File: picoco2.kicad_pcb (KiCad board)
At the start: 2 copper layers, 53.3 x 93.2 mm, 19 parts, among them J1 Conn_01x03_Female, Q1 Q_NMOS_GDS, SW1 SW_Push, SW2 SW_Push, U1 PicoW, U2 scd30, U3 ssd1306

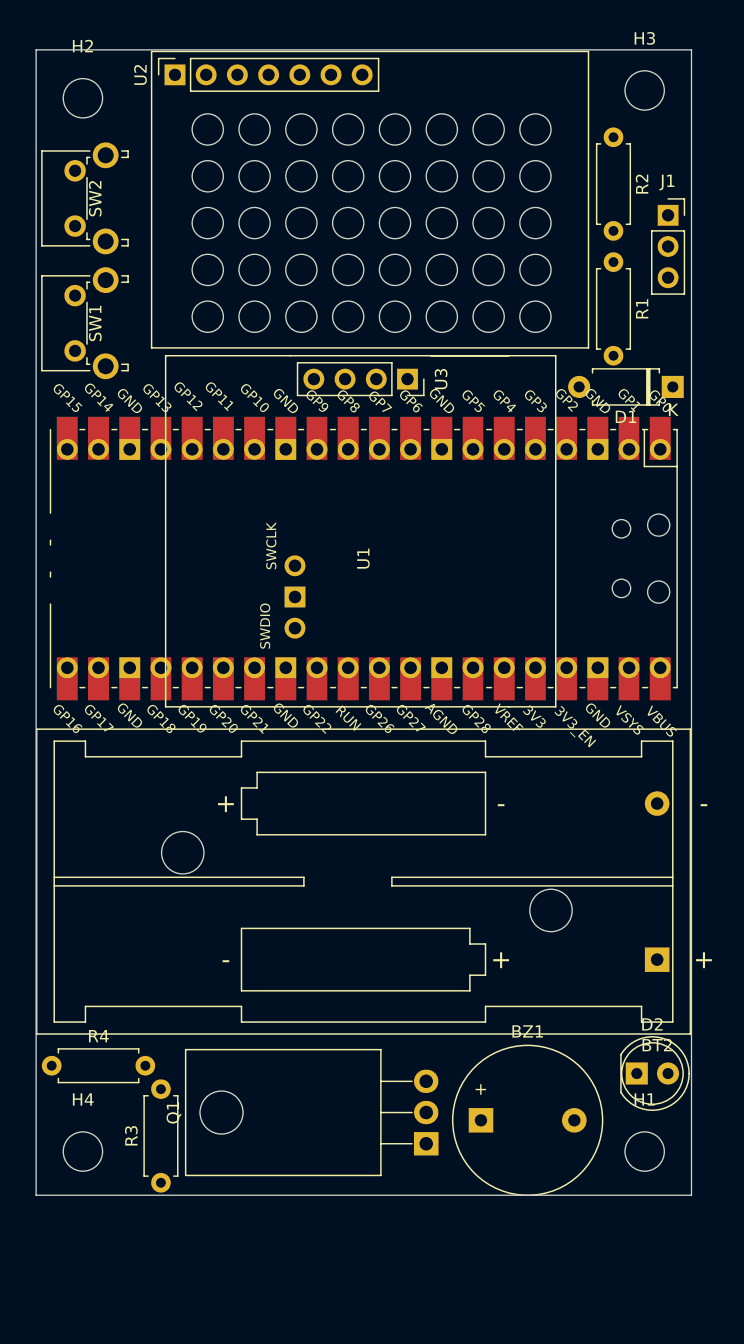
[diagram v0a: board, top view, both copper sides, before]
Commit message: update
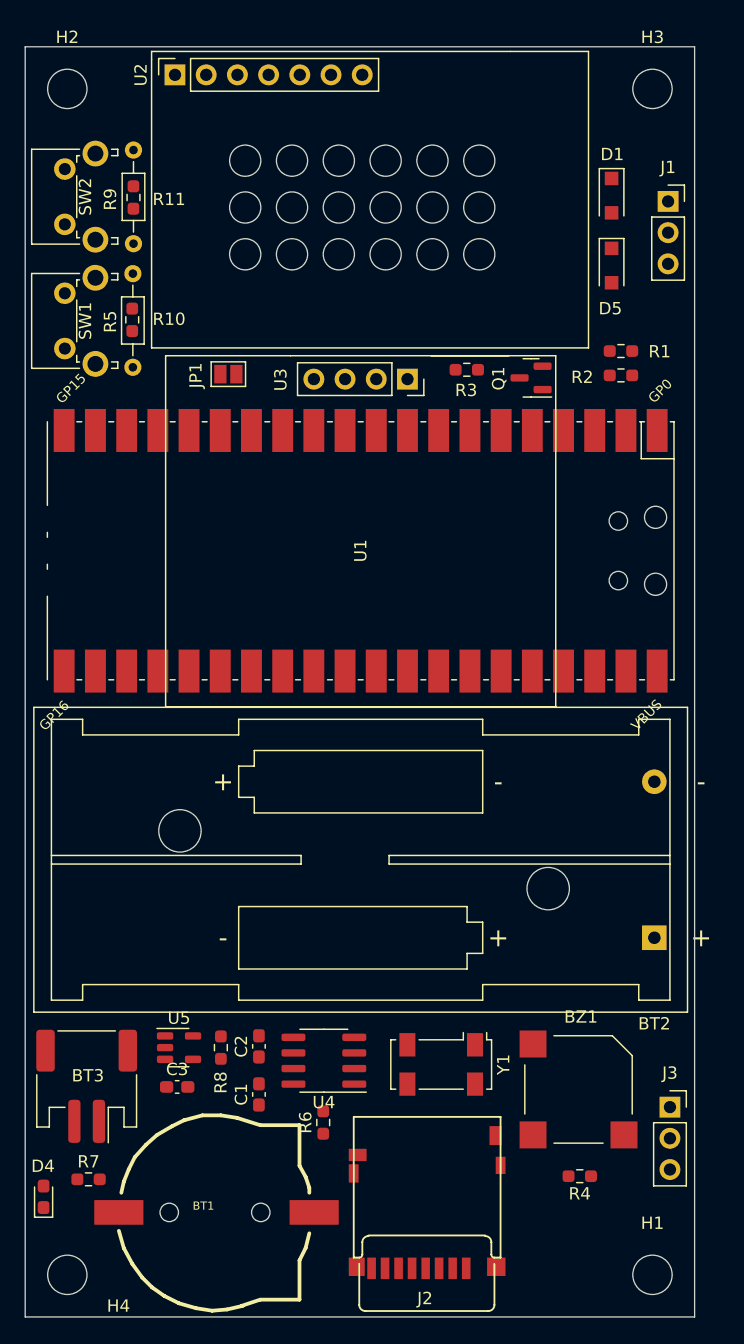
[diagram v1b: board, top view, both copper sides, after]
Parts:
- removed D2: LED, LED_THT:LED_D5.0mm
- added BT1: Battery, picoco2:CR1220-2, F.Cu at (109.6, 123.7)
- added BT3: Battery, Connector_JST:JST_PH_S2B-PH-SM4-TB_1x02-1MP_P2.00mm_Horizontal, F.Cu at (99.4, 113.4)
- added C1: C, Capacitor_SMD:C_0603_1608Metric_Pad1.08x0.95mm_HandSolder, F.Cu at (113.4, 114.1)
- added C2: C, Capacitor_SMD:C_0603_1608Metric_Pad1.08x0.95mm_HandSolder, F.Cu at (113.4, 110.2)
- added C3: C, Capacitor_SMD:C_0603_1608Metric_Pad1.08x0.95mm_HandSolder, F.Cu at (106.7, 113.5)
- added D4: LED, LED_SMD:LED_0603_1608Metric_Pad1.05x0.95mm_HandSolder, F.Cu at (95.9, 122.4)
- added D5: D, Diode_SMD:D_SOD-123F, F.Cu at (142.1, 46.6)
- added J2: Micro_SD_Card, picoco2:DM3D-SF_outline, F.Cu at (127.1, 127.4)
- added J3: Conn_01x03_Female, Connector_PinSocket_2.54mm:PinSocket_1x03_P2.54mm_Vertical, F.Cu at (146.8, 115.1)
- added JP1: SolderJumper_2_Open, Jumper:SolderJumper-2_P1.3mm_Open_Pad1.0x1.5mm, F.Cu at (110.9, 55.5)
- added R10: R, Resistor_THT:R_Axial_DIN0204_L3.6mm_D1.6mm_P7.62mm_Horizontal, F.Cu at (103.1, 54.9)
- added R11: R, Resistor_THT:R_Axial_DIN0204_L3.6mm_D1.6mm_P7.62mm_Horizontal, F.Cu at (103.2, 44.9)
- added R5: R, Resistor_SMD:R_0603_1608Metric_Pad0.98x0.95mm_HandSolder, F.Cu at (103.1, 51.1)
- added R6: R, Resistor_SMD:R_0603_1608Metric_Pad0.98x0.95mm_HandSolder, F.Cu at (118.6, 116.4)
- added R7: 1K, Resistor_SMD:R_0603_1608Metric_Pad0.98x0.95mm_HandSolder, F.Cu at (99.5, 121.0)
- added R8: 10K, Resistor_SMD:R_0603_1608Metric_Pad0.98x0.95mm_HandSolder, F.Cu at (110.3, 110.3)
- added R9: R, Resistor_SMD:R_0603_1608Metric_Pad0.98x0.95mm_HandSolder, F.Cu at (103.2, 41.1)
- added U4: PCF8523T, Package_SO:SOIC-8_3.9x4.9mm_P1.27mm, F.Cu at (118.7, 111.4)
- added U5: MCP73831-2-OT, Package_TO_SOT_SMD:SOT-23-5, F.Cu at (106.9, 110.3)
- added Y1: Crystal_GND23, Crystal:Crystal_SMD_Abracon_ABS25-4Pin_8.0x3.8mm, F.Cu at (128.2, 111.7)
- BZ1: footprint Buzzer_Beeper:Buzzer_12x9.5RM7.6 -> Buzzer_Beeper:MagneticBuzzer_Kobitone_254-EMB84Q-RO
- D1: footprint Diode_THT:D_A-405_P7.62mm_Horizontal -> Diode_SMD:D_SOD-123F
- Q1: footprint Package_TO_SOT_THT:TO-220-3_Horizontal_TabDown -> Package_TO_SOT_SMD:SOT-23
- R1, R2, R3, R4: footprint Resistor_THT:R_Axial_DIN0207_L6.3mm_D2.5mm_P7.62mm_Horizontal -> Resistor_SMD:R_0603_1608Metric_Pad0.98x0.95mm_HandSolder
- U1: footprint RPi_Pico:RPi_PicoW_SMD_TH -> RPi_Pico:RPi_PicoW_SMD
- moved R3 70.7 mm to (130.3, 55.1), turned to 0 degrees
- moved Q1 62.9 mm to (135.5, 55.8), turned to 180 degrees
- moved R4 43.9 mm to (139.5, 120.8), turned to 180 degrees
- moved R2 19.4 mm to (142.8, 55.6), turned to 180 degrees
- moved D1 16.3 mm to (142.1, 40.9), turned to -90 degrees
- moved H4 10.1 mm to (97.8, 128.8)
- moved H1 10.1 mm to (145.4, 128.8)
- moved BZ1 8.33 mm to (139.4, 113.7)
- moved R1 7.26 mm to (142.8, 53.6), turned to 180 degrees
- moved BT2 1.79 mm to (145.6, 101.3)
- moved H2 1.48 mm to (97.8, 32.3)
- moved J1 1.13 mm to (146.7, 41.4)
- moved SW1 0.86 mm to (97.6, 53.4)
- moved SW2 0.85 mm to (97.6, 43.3)
- moved U1 0.68 mm to (121.7, 69.8)
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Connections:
- BT2 pad 1: Net-(BT2-Pad1) -> VBAT_AAA
- BZ1 pad 1: unconnected-(BZ1-Pad1) -> BUZZER
- BZ1 pad 2: unconnected-(BZ1-Pad2) -> GND
- D1 pad 2: Net-(D1-Pad2) -> VBAT_AAA
- J1 pad 1: Net-(D1-Pad2) -> VSYS
- J1 pad 2: Net-(BT2-Pad1) -> Net-(D1-Pad1)
- J1 pad 3: unconnected-(J1-Pad3) -> Net-(J1-Pad3)
- Q1 pad 1: unconnected-(Q1-Pad1) -> SCD30_EN
- Q1 pad 2: unconnected-(Q1-Pad2) -> SCD30_GND
- Q1 pad 3: unconnected-(Q1-Pad3) -> GND
- R1 pad 2: Net-(R1-Pad2) -> SDA
- R2 pad 2: Net-(R2-Pad2) -> SCL
- R3 pad 1: unconnected-(R3-Pad1) -> SCD30_EN
- R3 pad 2: unconnected-(R3-Pad2) -> GND
- R4 pad 1: unconnected-(R4-Pad1) -> Net-(J3-Pad2)
- R4 pad 2: unconnected-(R4-Pad2) -> GND
- SW1 pad 1: unconnected-(SW1-Pad1) -> BUT_A
- SW1 pad 2: unconnected-(SW1-Pad2) -> GND
- SW2 pad 1: unconnected-(SW2-Pad1) -> BUT_B
- SW2 pad 2: unconnected-(SW2-Pad2) -> GND
- U1 pad 1: unconnected-(U1-Pad1) -> SDA
- U1 pad 14: unconnected-(U1-Pad14) -> SCK
- U1 pad 15: unconnected-(U1-Pad15) -> MOSI
- U1 pad 16: unconnected-(U1-Pad16) -> MISO
- U1 pad 2: unconnected-(U1-Pad2) -> SCL
- U1 pad 26: Net-(R2-Pad2) -> unconnected-(U1-Pad26)
- U1 pad 27: Net-(R1-Pad2) -> unconnected-(U1-Pad27)
- U1 pad 39: Net-(D1-Pad1) -> VSYS
- U1 pad 4: unconnected-(U1-Pad4) -> SD_CS
- U1 pad 40: unconnected-(U1-Pad40) -> VBUS
- U2 pad 2: GND -> SCD30_GND
- U2 pad 3: Net-(R1-Pad2) -> SCL
- U2 pad 4: Net-(R2-Pad2) -> SCL
- U3 pad 3: Net-(R1-Pad2) -> SCL
- U3 pad 4: Net-(R2-Pad2) -> SCL
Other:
- board size 53.3 x 93.2 mm -> 54.5 x 103.4 mm

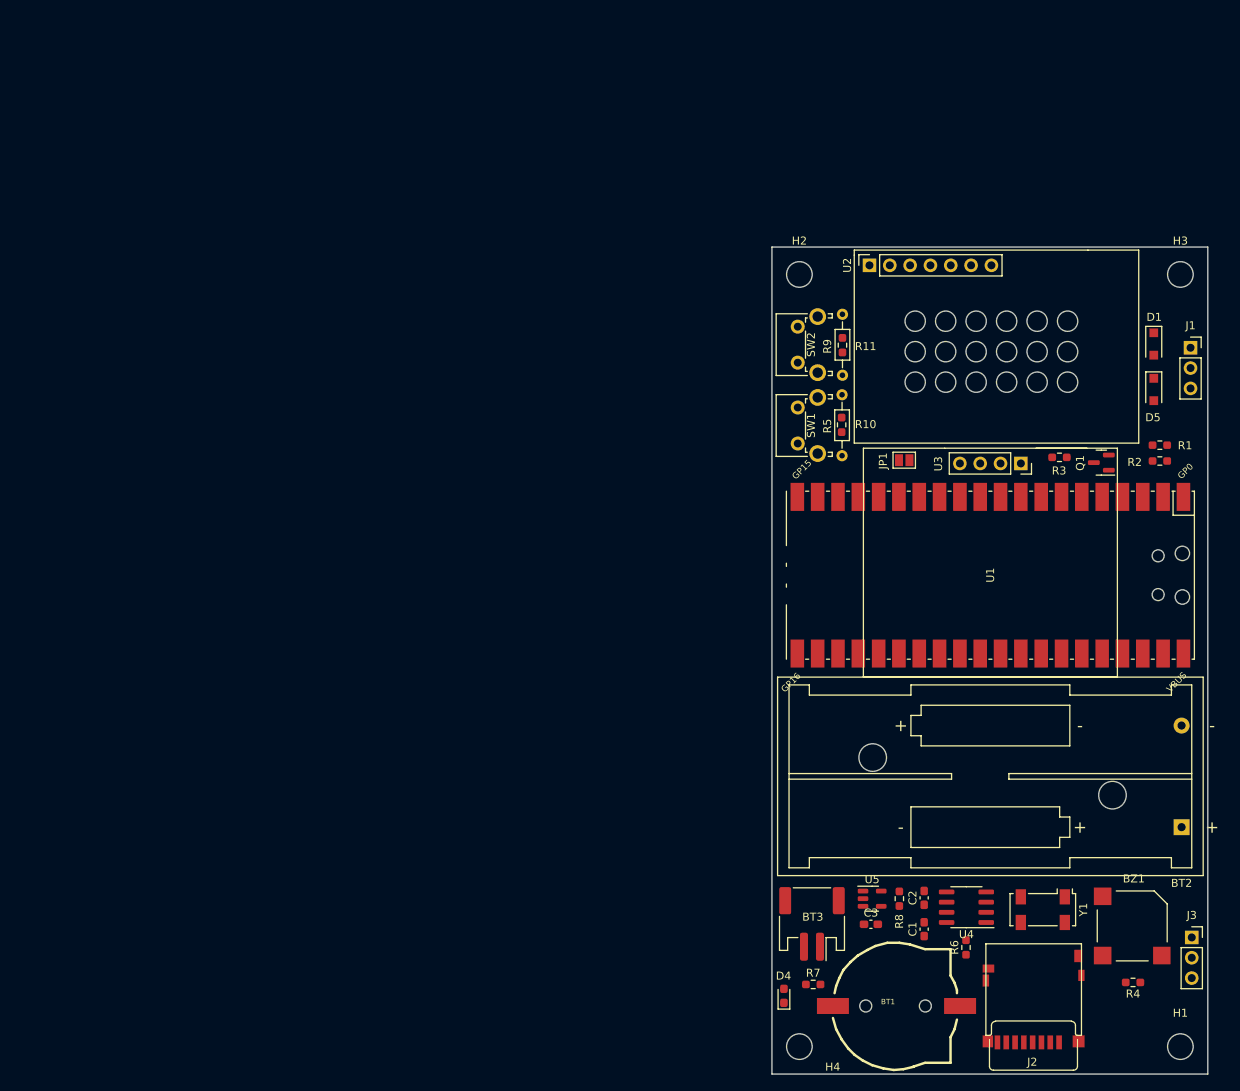
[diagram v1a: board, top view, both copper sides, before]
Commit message: basic layout done
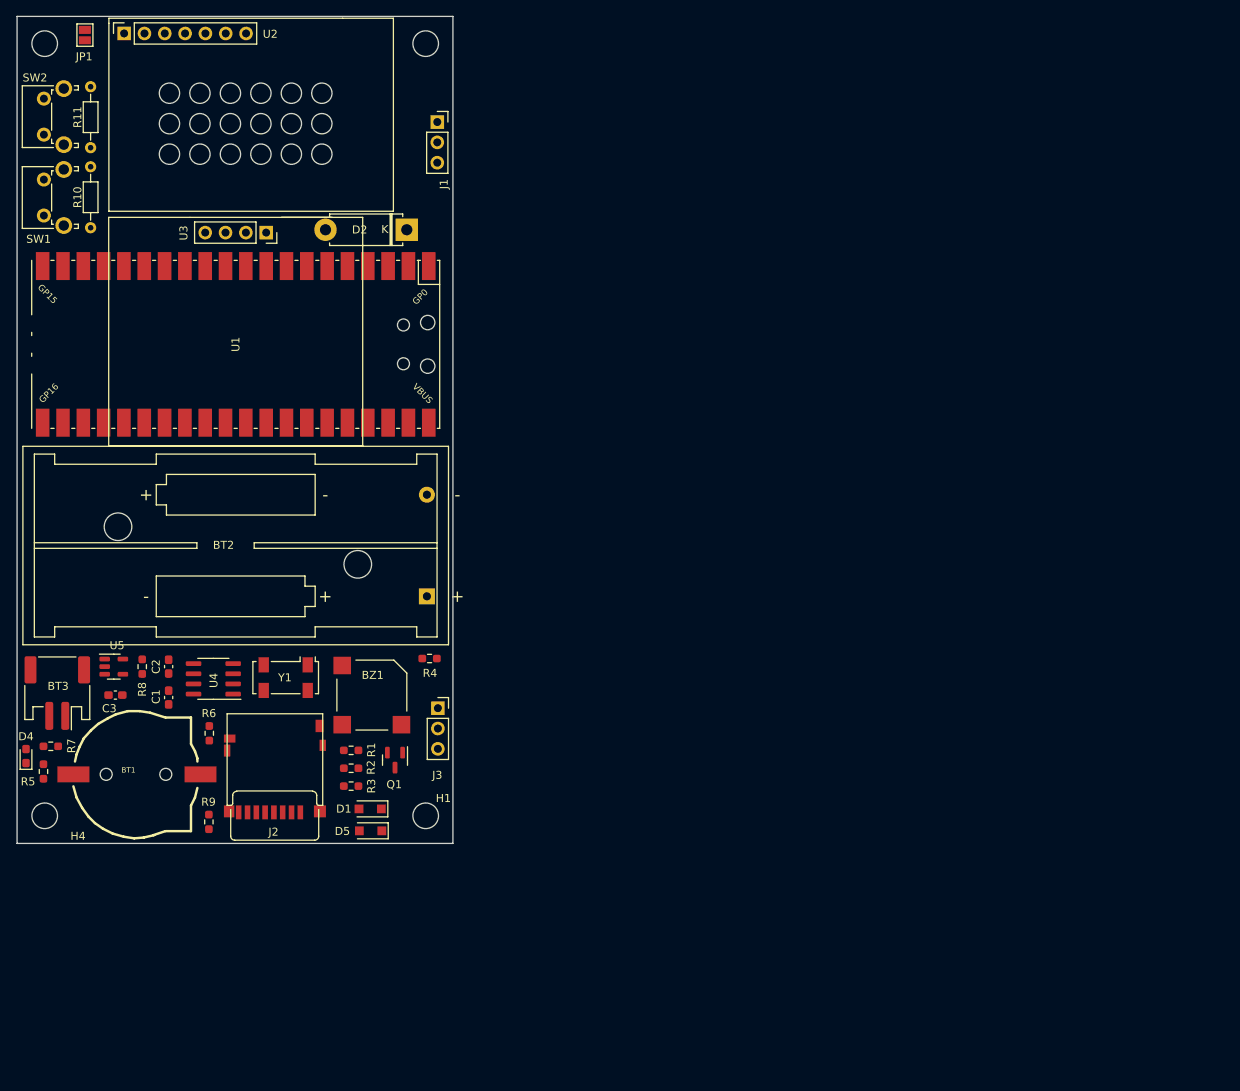
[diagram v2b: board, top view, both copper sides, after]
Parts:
- added D2: D, Diode_THT:D_5W_P10.16mm_Horizontal, F.Cu at (48.7, 26.7)
- moved JP1 115.4 mm to (8.48, 2.34), turned to 90 degrees
- moved D1 113.9 mm to (44.1, 99.1), turned to 180 degrees
- moved D5 112.4 mm to (44.2, 101.8), turned to 180 degrees
- moved R5 108.8 mm to (3.30, 94.4)
- moved R2 108.1 mm to (41.8, 94.0)
- moved R1 108.1 mm to (41.8, 91.7)
- moved R7 99.8 mm to (4.22, 91.2)
- moved D4 99.4 mm to (1.12, 92.5)
- moved BZ1 99.3 mm to (44.3, 84.8)
- moved BT1 99.3 mm to (14.6, 94.7)
- moved U5 99.1 mm to (12.1, 81.3)
- moved R9 99.1 mm to (24.0, 100.7)
- moved J2 99.1 mm to (32.2, 98.6)
- moved R8 99.0 mm to (15.6, 81.3)
- moved Y1 99.0 mm to (33.6, 82.7)
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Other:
- outline, holes or cut-outs redrawn
